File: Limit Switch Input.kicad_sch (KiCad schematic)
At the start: 4 parts

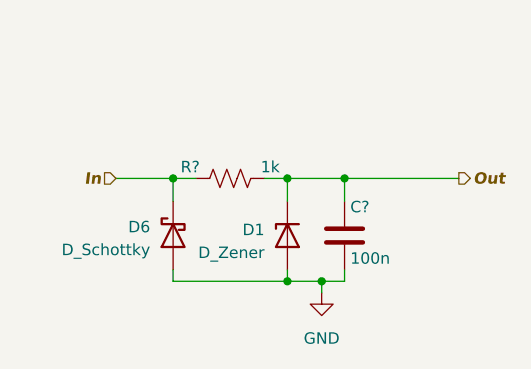
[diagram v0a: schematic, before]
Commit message: Ready for design review
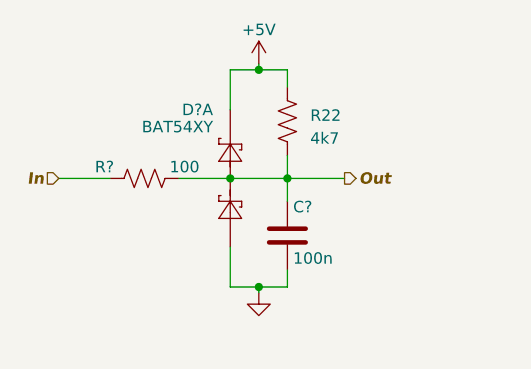
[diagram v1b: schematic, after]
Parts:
- removed D1: D_Zener, Diode_SMD:D_SOD-523, symbol Device:D_Zener
- removed D6: D_Schottky, Diode_SMD:D_SOD-523, symbol Device:D_Schottky
- added D?: BAT54XY, Package_TO_SOT_SMD:SOT-363_SC-70-6, symbol Diode:BAT54SW
- added R22: 4k7, Resistor_SMD:R_0402_1005Metric, symbol Device:R_US
- C?: DigiKey 490-10700-1-ND -> 490-3261-1-ND; LCSC (none) -> C71629
- R?: value 1k -> 100; DigiKey 311-1.00KLRCT-ND -> 311-100JRCT-ND; LCSC (none) -> C106233
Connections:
- net GND: now also D?.1 (A)
- net Out: now also D?.6 (COM), R22.2
- new net +5V: D?.2 (K), R22.1
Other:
- moved on the sheet: C?, R?

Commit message: Update
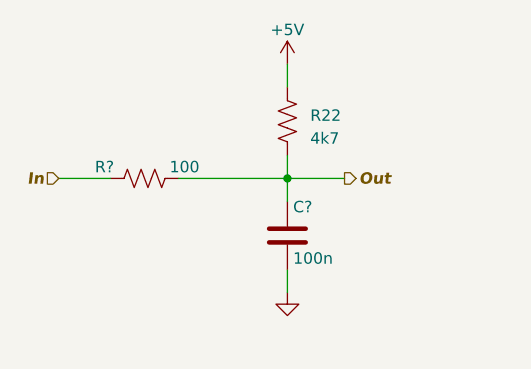
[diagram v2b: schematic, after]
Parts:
- removed D?: BAT54XY, Package_TO_SOT_SMD:SOT-363_SC-70-6, symbol Diode:BAT54SW
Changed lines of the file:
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@@
     (comment 4 "S. Bywater")
   )
-  (junction (at 127 76.2) (diameter 0) (color 0 0 0 0)
-  )
-  (junction (at 130.175 88.265) (diameter 0) (color 0 0 0 0)
-  )
   (junction (at 133.35 76.2) (diameter 0) (color 0 0 0 0)
   )
-  (junction (at 130.175 64.135) (diameter 0) (color 0 0 0 0)
-  )
-  (wire (pts (xy 127 64.135) (xy 130.175 64.135))
-    (stroke (width 0) (type default))
-  )
   (wire (pts (xy 133.35 76.2) (xy 139.7 76.2))
     (stroke (width 0) (type default))
@@
     (stroke (width 0) (type default))
   )
-  (wire (pts (xy 121.285 76.2) (xy 127 76.2))
-    (stroke (width 0) (type default))
-  )
-  (wire (pts (xy 130.175 63.5) (xy 130.175 64.135))
+  (wire (pts (xy 121.285 76.2) (xy 133.35 76.2))
+    (stroke (width 0) (type default))
+  )
+  (wire (pts (xy 133.35 63.5) (xy 133.35 66.04))
     (stroke (width 0) (type default))
   )
@@
     (stroke (width 0) (type default))
   )
-  (wire (pts (xy 130.175 64.135) (xy 133.35 64.135))
-    (stroke (width 0) (type default))
-  )
-  (wire (pts (xy 130.175 88.265) (xy 133.35 88.265))
-    (stroke (width 0) (type default))
-  )
-  (wire (pts (xy 130.175 88.265) (xy 130.175 88.9))
-    (stroke (width 0) (type default))
-  )
   (wire (pts (xy 107.95 76.2) (xy 113.665 76.2))
     (stroke (width 0) (type default))
   )
-  (wire (pts (xy 130.175 88.265) (xy 127 88.265))
-    (stroke (width 0) (type default))
-  )
-  (wire (pts (xy 127 88.265) (xy 127 83.82))
-    (stroke (width 0) (type default))
-  )
-  (wire (pts (xy 133.35 88.265) (xy 133.35 86.36))
-    (stroke (width 0) (type default))
-  )
-  (wire (pts (xy 127 76.2) (xy 133.35 76.2))
-    (stroke (width 0) (type default))
-  )
-  (wire (pts (xy 133.35 64.135) (xy 133.35 66.04))
-    (stroke (width 0) (type default))
-  )
-  (wire (pts (xy 127 68.58) (xy 127 64.135))
+  (wire (pts (xy 133.35 86.36) (xy 133.35 88.9))
     (stroke (width 0) (type default))
   )
@@
           (reference "R24") (unit 1)
         )
-        (path "/6b38a626-de8c-4b2d-bc76-3a02bc823a86/3c576bdf-2a9b-47b5-bf2f-8d65e4282c90"
-          (reference "R26") (unit 1)
-        )
-      )
-    )
-  )
-  (symbol (lib_id "power:GND") (at 130.175 88.9 0) (unit 1)
+      )
+    )
+  )
+  (symbol (lib_id "power:GND") (at 133.35 88.9 0) (unit 1)
     (in_bom yes) (on_board yes) (dnp no) (fields_autoplaced)
-    (property "Reference" "#PWR010" (at 130.175 95.25 0)
-      (effects (font (size 1.27 1.27)) hide)
-    )
-    (property "Value" "GND" (at 130.175 93.98 0)
-      (effects (font (size 1.27 1.27)) hide)
-    )
-    (property "Footprint" "" (at 130.175 88.9 0)
-      (effects (font (size 1.27 1.27)) hide)
-    )
-    (property "Datasheet" "" (at 130.175 88.9 0)
+    (property "Reference" "#PWR010" (at 133.35 95.25 0)
+      (effects (font (size 1.27 1.27)) hide)
+    )
+    (property "Value" "GND" (at 133.35 93.98 0)
+      (effects (font (size 1.27 1.27)) hide)
+    )
+    (property "Footprint" "" (at 133.35 88.9 0)
+      (effects (font (size 1.27 1.27)) hide)
+    )
+    (property "Datasheet" "" (at 133.35 88.9 0)
       (effects (font (size 1.27 1.27)) hide)
     )
@@
         (path "/6b38a626-de8c-4b2d-bc76-3a02bc823a86/5fa307ae-0220-4647-a069-86a82689cac4"
           (reference "#PWR014") (unit 1)
-        )
-        (path "/6b38a626-de8c-4b2d-bc76-3a02bc823a86/3c576bdf-2a9b-47b5-bf2f-8d65e4282c90"
-          (reference "#PWR016") (unit 1)
-        )
-      )
-    )
-  )
-  (symbol (lib_id "Diode:BAT54SW") (at 127 76.2 90) (unit 1)
-    (in_bom yes) (on_board yes) (dnp no)
-    (property "Reference" "D?" (at 125.095 68.58 90)
-      (effects (font (size 1.27 1.27)) (justify left))
-    )
-    (property "Value" "BAT54XY" (at 125.095 70.485 90)
-      (effects (font (size 1.27 1.27)) (justify left))
-    )
-    (property "Footprint" "Package_TO_SOT_SMD:SOT-363_SC-70-6" (at 130.81 76.2 0)
-      (effects (font (size 1.27 1.27)) (justify left) hide)
-    )
-    (property "Datasheet" "https://assets.nexperia.com/documents/data-sheet/BAT54W_SER.pdf" (at 130.81 76.2 0)
-      (effects (font (size 1.27 1.27)) hide)
-    )
-    (property "LCSC" "C282367" (at 127 76.2 0)
-      (effects (font (size 1.27 1.27)) hide)
-    )
-    (property "DigiKey" "1727-3571-1-ND" (at 127 76.2 0)
-      (effects (font (size 1.27 1.27)) hide)
-    )
-    (pin "1")
-    (pin "2")
-    (pin "6")
-    (pin "3")
-    (pin "4")
-    (pin "5")
-    (instances
-      (project "ECE4760 Motor Driver"
-        (path "/6b38a626-de8c-4b2d-bc76-3a02bc823a86"
-          (reference "D?") (unit 1)
-        )
-        (path "/6b38a626-de8c-4b2d-bc76-3a02bc823a86/9895140f-573d-481d-a8a6-67e4fef141c0"
-          (reference "D3") (unit 1)
-        )
-        (path "/6b38a626-de8c-4b2d-bc76-3a02bc823a86/299487ec-ee2d-43f4-ae82-35783d2e6b45"
-          (reference "D3") (unit 2)
-        )
-        (path "/6b38a626-de8c-4b2d-bc76-3a02bc823a86/5fa307ae-0220-4647-a069-86a82689cac4"
-          (reference "D4") (unit 1)
-        )
-        (path "/6b38a626-de8c-4b2d-bc76-3a02bc823a86/3c576bdf-2a9b-47b5-bf2f-8d65e4282c90"
-          (reference "D4") (unit 2)
         )
       )
@@
           (reference "R25") (unit 1)
         )
-        (path "/6b38a626-de8c-4b2d-bc76-3a02bc823a86/3c576bdf-2a9b-47b5-bf2f-8d65e4282c90"
-          (reference "R27") (unit 1)
-        )
-      )
-    )
-  )
-  (symbol (lib_id "power:+5V") (at 130.175 63.5 0) (unit 1)
+      )
+    )
+  )
+  (symbol (lib_id "power:+5V") (at 133.35 63.5 0) (unit 1)
     (in_bom yes) (on_board yes) (dnp no) (fields_autoplaced)
-    (property "Reference" "#PWR011" (at 130.175 67.31 0)
-      (effects (font (size 1.27 1.27)) hide)
-    )
-    (property "Value" "+5V" (at 130.175 59.69 0)
+    (property "Reference" "#PWR011" (at 133.35 67.31 0)
+      (effects (font (size 1.27 1.27)) hide)
+    )
+    (property "Value" "+5V" (at 133.35 59.69 0)
       (effects (font (size 1.27 1.27)))
     )
-    (property "Footprint" "" (at 130.175 63.5 0)
-      (effects (font (size 1.27 1.27)) hide)
-    )
-    (property "Datasheet" "" (at 130.175 63.5 0)
+    (property "Footprint" "" (at 133.35 63.5 0)
+      (effects (font (size 1.27 1.27)) hide)
+    )
+    (property "Datasheet" "" (at 133.35 63.5 0)
       (effects (font (size 1.27 1.27)) hide)
     )
@@
         (path "/6b38a626-de8c-4b2d-bc76-3a02bc823a86/5fa307ae-0220-4647-a069-86a82689cac4"
           (reference "#PWR013") (unit 1)
-        )
-        (path "/6b38a626-de8c-4b2d-bc76-3a02bc823a86/3c576bdf-2a9b-47b5-bf2f-8d65e4282c90"
-          (reference "#PWR015") (unit 1)
         )
       )
@@
           (reference "C67") (unit 1)
         )
-        (path "/6b38a626-de8c-4b2d-bc76-3a02bc823a86/3c576bdf-2a9b-47b5-bf2f-8d65e4282c90"
-          (reference "C68") (unit 1)
-        )
-      )
+      )
